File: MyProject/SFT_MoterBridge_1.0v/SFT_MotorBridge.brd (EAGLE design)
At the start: 100 x 65 mm, 44 parts

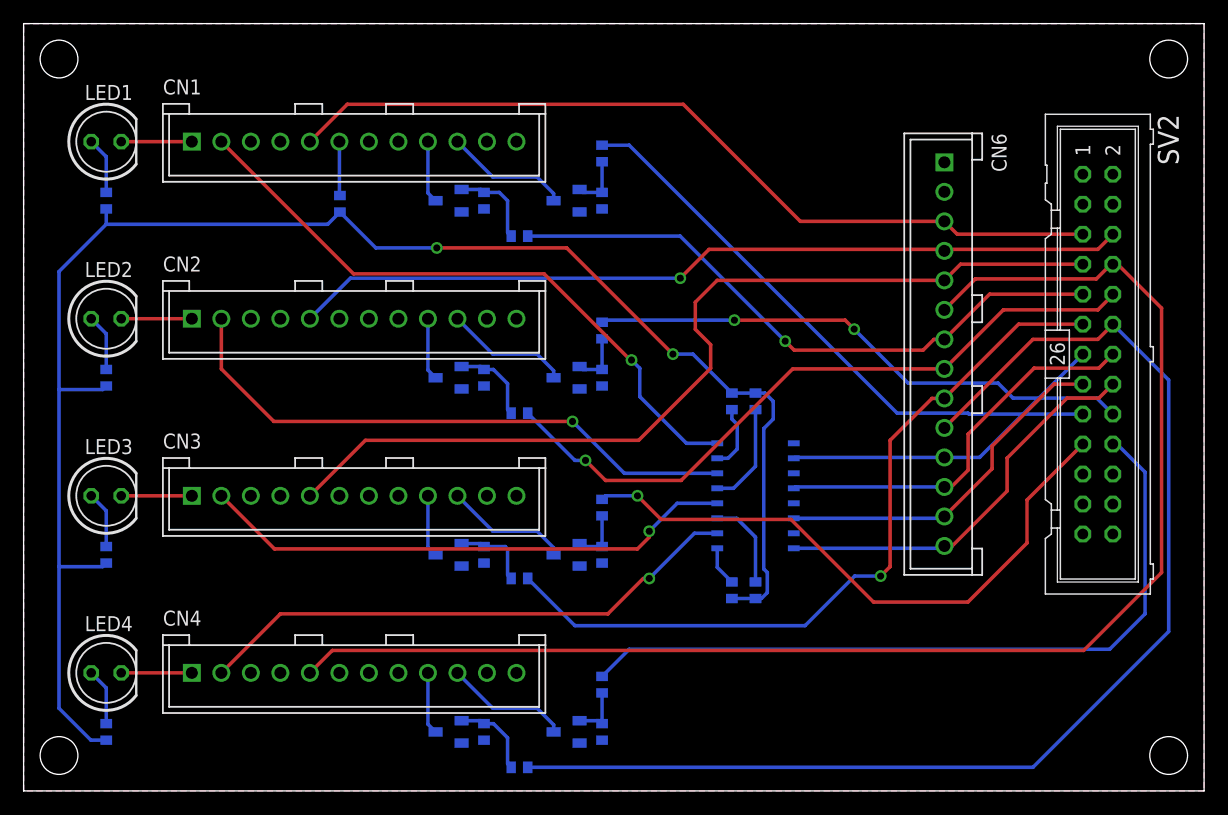
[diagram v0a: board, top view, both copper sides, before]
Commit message: kyuukei reset
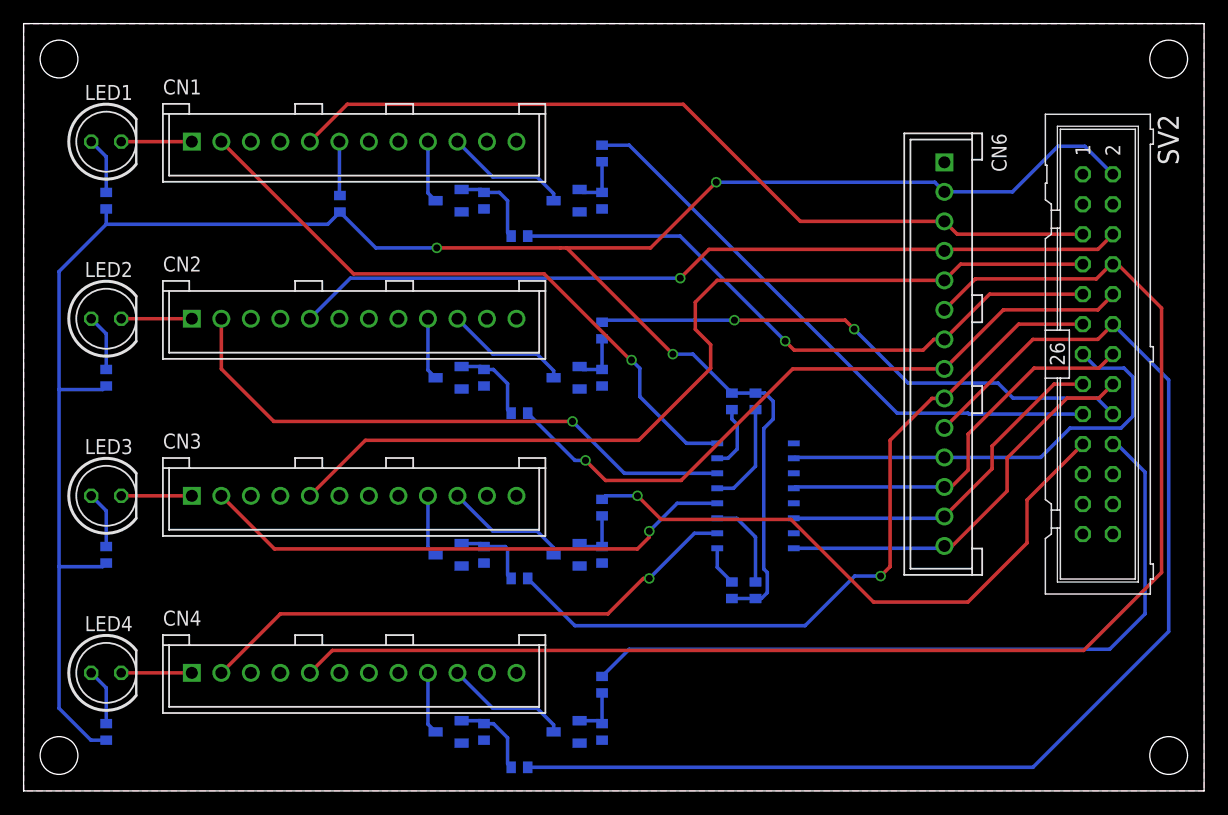
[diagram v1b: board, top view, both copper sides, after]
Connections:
- net +5V: now also CN6.2, SV2.2
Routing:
- net +5V: track 140.8 -> 192.3 mm, vias 2 -> 3
- net SPEED_OUT_1: track 28.1 -> 38.6 mm

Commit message: tetuya
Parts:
- added DRILEGEND: (no value), drilegend:DRILEGEND
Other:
- board text added: "穴図"

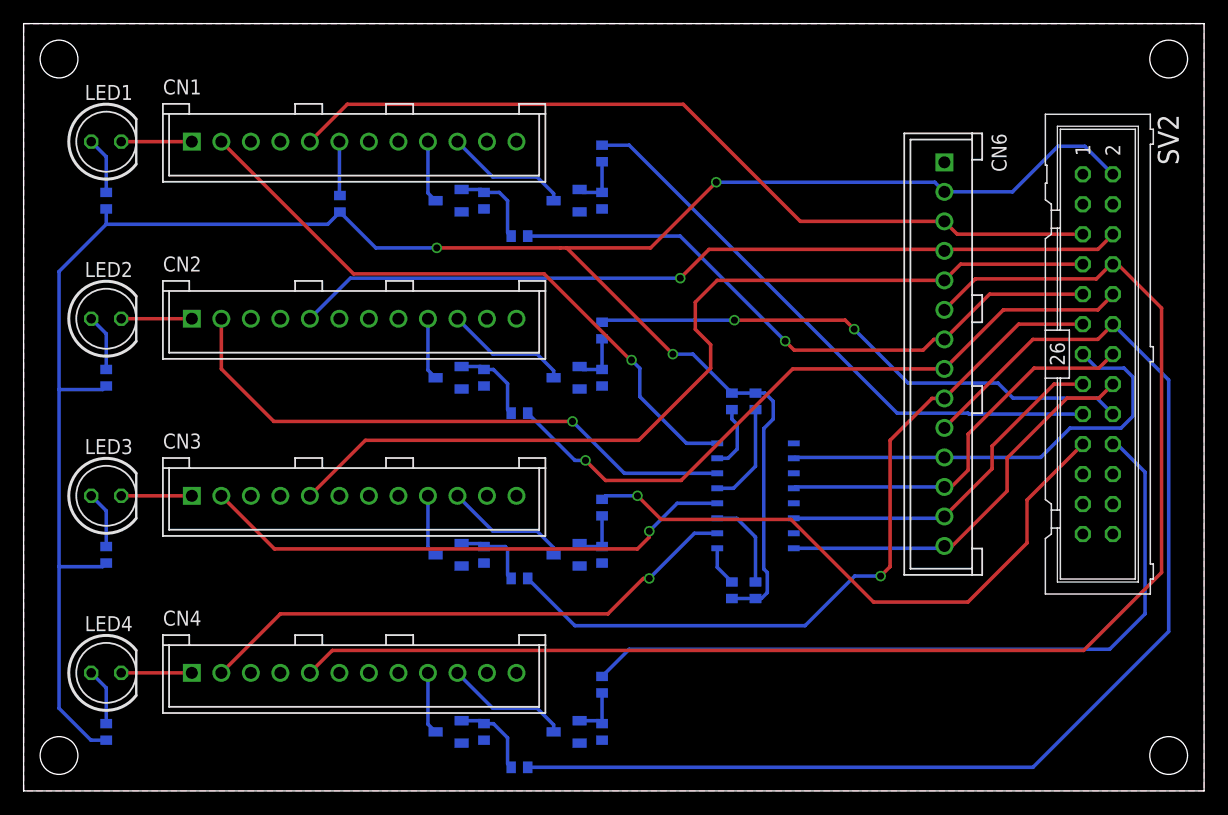
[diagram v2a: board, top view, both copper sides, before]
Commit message: test2
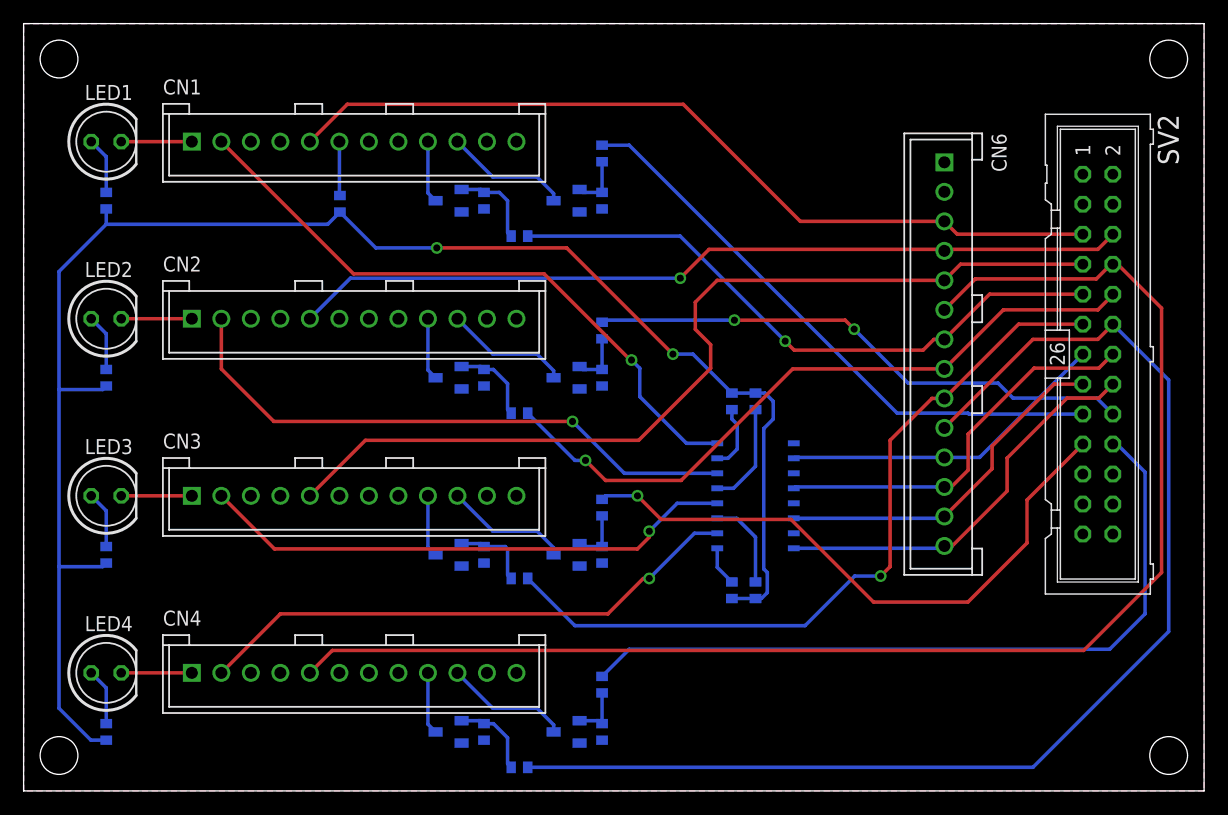
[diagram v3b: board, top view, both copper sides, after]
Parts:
- removed DRILEGEND: (no value), drilegend:DRILEGEND
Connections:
- net +5V: no longer CN6.2, SV2.2
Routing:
- net +5V: track 192.3 -> 140.8 mm, vias 3 -> 2
- net SPEED_OUT_1: track 38.6 -> 28.1 mm
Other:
- board text removed: "穴図"
